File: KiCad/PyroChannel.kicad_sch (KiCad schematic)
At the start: 5 parts, among them Q4 IRLML0030

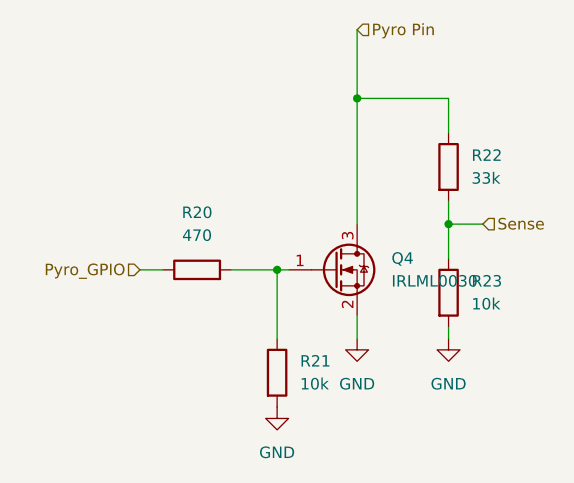
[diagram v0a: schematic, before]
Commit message: Layout started
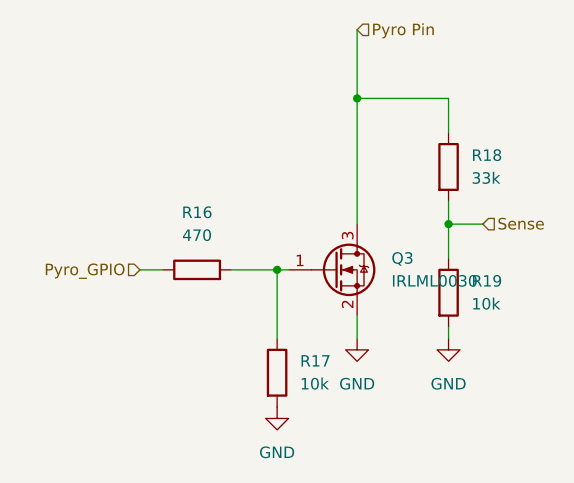
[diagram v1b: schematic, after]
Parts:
- renumbered Q4 to Q3, R20 to R16, R21 to R17, R22 to R18, R23 to R19
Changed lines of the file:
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@@
 		(dnp no)
 		(fields_autoplaced yes)
-		(property "Reference" "#PWR072"
+		(property "Reference" "#PWR069"
 			(at 157.48 107.95 0)
 			(effects
@@
 		(instances
 			(project "Senior Project"
-				(path "/16f8cce7-467e-4342-b55a-00af81cd6f69/4f56c78f-4532-4c9f-be6c-2bbf693c5fca"
+				(path "/16f8cce7-467e-4342-b55a-00af81cd6f69/553e2c15-6dd9-455d-b91b-1c20c70d481b"
+					(reference "#PWR066")
+					(unit 1)
+				)
+				(path "/16f8cce7-467e-4342-b55a-00af81cd6f69/60268ff6-e480-4c50-9139-8340585ef982"
+					(reference "#PWR069")
+					(unit 1)
+				)
+				(path "/16f8cce7-467e-4342-b55a-00af81cd6f69/93da445a-87ee-42db-a7a9-6194d5b9218b"
 					(reference "#PWR072")
-					(unit 1)
-				)
-				(path "/16f8cce7-467e-4342-b55a-00af81cd6f69/528e247e-1625-48b4-9899-73b4b85367ce"
-					(reference "#PWR069")
-					(unit 1)
-				)
-				(path "/16f8cce7-467e-4342-b55a-00af81cd6f69/553e2c15-6dd9-455d-b91b-1c20c70d481b"
-					(reference "#PWR066")
 					(unit 1)
 				)
@@
 		(dnp no)
 		(fields_autoplaced yes)
-		(property "Reference" "#PWR071"
+		(property "Reference" "#PWR068"
 			(at 147.32 107.95 0)
 			(effects
@@
 		(instances
 			(project "Senior Project"
-				(path "/16f8cce7-467e-4342-b55a-00af81cd6f69/4f56c78f-4532-4c9f-be6c-2bbf693c5fca"
+				(path "/16f8cce7-467e-4342-b55a-00af81cd6f69/553e2c15-6dd9-455d-b91b-1c20c70d481b"
+					(reference "#PWR057")
+					(unit 1)
+				)
+				(path "/16f8cce7-467e-4342-b55a-00af81cd6f69/60268ff6-e480-4c50-9139-8340585ef982"
+					(reference "#PWR068")
+					(unit 1)
+				)
+				(path "/16f8cce7-467e-4342-b55a-00af81cd6f69/93da445a-87ee-42db-a7a9-6194d5b9218b"
 					(reference "#PWR071")
-					(unit 1)
-				)
-				(path "/16f8cce7-467e-4342-b55a-00af81cd6f69/528e247e-1625-48b4-9899-73b4b85367ce"
-					(reference "#PWR068")
-					(unit 1)
-				)
-				(path "/16f8cce7-467e-4342-b55a-00af81cd6f69/553e2c15-6dd9-455d-b91b-1c20c70d481b"
-					(reference "#PWR057")
 					(unit 1)
 				)
@@
 		(dnp no)
 		(fields_autoplaced yes)
-		(property "Reference" "R22"
+		(property "Reference" "R18"
 			(at 160.02 81.2799 0)
 			(effects
@@
 		(instances
 			(project "Senior Project"
-				(path "/16f8cce7-467e-4342-b55a-00af81cd6f69/4f56c78f-4532-4c9f-be6c-2bbf693c5fca"
+				(path "/16f8cce7-467e-4342-b55a-00af81cd6f69/553e2c15-6dd9-455d-b91b-1c20c70d481b"
+					(reference "R14")
+					(unit 1)
+				)
+				(path "/16f8cce7-467e-4342-b55a-00af81cd6f69/60268ff6-e480-4c50-9139-8340585ef982"
+					(reference "R18")
+					(unit 1)
+				)
+				(path "/16f8cce7-467e-4342-b55a-00af81cd6f69/93da445a-87ee-42db-a7a9-6194d5b9218b"
 					(reference "R22")
-					(unit 1)
-				)
-				(path "/16f8cce7-467e-4342-b55a-00af81cd6f69/528e247e-1625-48b4-9899-73b4b85367ce"
-					(reference "R18")
-					(unit 1)
-				)
-				(path "/16f8cce7-467e-4342-b55a-00af81cd6f69/553e2c15-6dd9-455d-b91b-1c20c70d481b"
-					(reference "R14")
 					(unit 1)
 				)
@@
 		(dnp no)
 		(fields_autoplaced yes)
-		(property "Reference" "#PWR070"
+		(property "Reference" "#PWR067"
 			(at 138.43 115.57 0)
 			(effects
@@
 		(instances
 			(project "Senior Project"
-				(path "/16f8cce7-467e-4342-b55a-00af81cd6f69/4f56c78f-4532-4c9f-be6c-2bbf693c5fca"
+				(path "/16f8cce7-467e-4342-b55a-00af81cd6f69/553e2c15-6dd9-455d-b91b-1c20c70d481b"
+					(reference "#PWR056")
+					(unit 1)
+				)
+				(path "/16f8cce7-467e-4342-b55a-00af81cd6f69/60268ff6-e480-4c50-9139-8340585ef982"
+					(reference "#PWR067")
+					(unit 1)
+				)
+				(path "/16f8cce7-467e-4342-b55a-00af81cd6f69/93da445a-87ee-42db-a7a9-6194d5b9218b"
 					(reference "#PWR070")
-					(unit 1)
-				)
-				(path "/16f8cce7-467e-4342-b55a-00af81cd6f69/528e247e-1625-48b4-9899-73b4b85367ce"
-					(reference "#PWR067")
-					(unit 1)
-				)
-				(path "/16f8cce7-467e-4342-b55a-00af81cd6f69/553e2c15-6dd9-455d-b91b-1c20c70d481b"
-					(reference "#PWR056")
 					(unit 1)
 				)
@@
 		(dnp no)
 		(fields_autoplaced yes)
-		(property "Reference" "R20"
+		(property "Reference" "R16"
 			(at 129.54 87.63 90)
 			(effects
@@
 		(instances
 			(project "Senior Project"
-				(path "/16f8cce7-467e-4342-b55a-00af81cd6f69/4f56c78f-4532-4c9f-be6c-2bbf693c5fca"
+				(path "/16f8cce7-467e-4342-b55a-00af81cd6f69/553e2c15-6dd9-455d-b91b-1c20c70d481b"
+					(reference "R12")
+					(unit 1)
+				)
+				(path "/16f8cce7-467e-4342-b55a-00af81cd6f69/60268ff6-e480-4c50-9139-8340585ef982"
+					(reference "R16")
+					(unit 1)
+				)
+				(path "/16f8cce7-467e-4342-b55a-00af81cd6f69/93da445a-87ee-42db-a7a9-6194d5b9218b"
 					(reference "R20")
-					(unit 1)
-				)
-				(path "/16f8cce7-467e-4342-b55a-00af81cd6f69/528e247e-1625-48b4-9899-73b4b85367ce"
-					(reference "R16")
-					(unit 1)
-				)
-				(path "/16f8cce7-467e-4342-b55a-00af81cd6f69/553e2c15-6dd9-455d-b91b-1c20c70d481b"
-					(reference "R12")
 					(unit 1)
 				)
@@
 		(dnp no)
 		(fields_autoplaced yes)
-		(property "Reference" "Q4"
+		(property "Reference" "Q3"
 			(at 151.13 92.7099 0)
 			(effects
@@
 		(instances
 			(project "Senior Project"
-				(path "/16f8cce7-467e-4342-b55a-00af81cd6f69/4f56c78f-4532-4c9f-be6c-2bbf693c5fca"
+				(path "/16f8cce7-467e-4342-b55a-00af81cd6f69/553e2c15-6dd9-455d-b91b-1c20c70d481b"
+					(reference "Q2")
+					(unit 1)
+				)
+				(path "/16f8cce7-467e-4342-b55a-00af81cd6f69/60268ff6-e480-4c50-9139-8340585ef982"
+					(reference "Q3")
+					(unit 1)
+				)
+				(path "/16f8cce7-467e-4342-b55a-00af81cd6f69/93da445a-87ee-42db-a7a9-6194d5b9218b"
 					(reference "Q4")
-					(unit 1)
-				)
-				(path "/16f8cce7-467e-4342-b55a-00af81cd6f69/528e247e-1625-48b4-9899-73b4b85367ce"
-					(reference "Q3")
-					(unit 1)
-				)
-				(path "/16f8cce7-467e-4342-b55a-00af81cd6f69/553e2c15-6dd9-455d-b91b-1c20c70d481b"
-					(reference "Q2")
 					(unit 1)
 				)
@@
 		(dnp no)
 		(fields_autoplaced yes)
-		(property "Reference" "R21"
+		(property "Reference" "R17"
 			(at 140.97 104.1399 0)
 			(effects
@@
 		(instances
 			(project "Senior Project"
-				(path "/16f8cce7-467e-4342-b55a-00af81cd6f69/4f56c78f-4532-4c9f-be6c-2bbf693c5fca"
+				(path "/16f8cce7-467e-4342-b55a-00af81cd6f69/553e2c15-6dd9-455d-b91b-1c20c70d481b"
+					(reference "R13")
+					(unit 1)
+				)
+				(path "/16f8cce7-467e-4342-b55a-00af81cd6f69/60268ff6-e480-4c50-9139-8340585ef982"
+					(reference "R17")
+					(unit 1)
+				)
+				(path "/16f8cce7-467e-4342-b55a-00af81cd6f69/93da445a-87ee-42db-a7a9-6194d5b9218b"
 					(reference "R21")
-					(unit 1)
-				)
-				(path "/16f8cce7-467e-4342-b55a-00af81cd6f69/528e247e-1625-48b4-9899-73b4b85367ce"
-					(reference "R17")
-					(unit 1)
-				)
-				(path "/16f8cce7-467e-4342-b55a-00af81cd6f69/553e2c15-6dd9-455d-b91b-1c20c70d481b"
-					(reference "R13")
 					(unit 1)
 				)
@@
 		(dnp no)
 		(fields_autoplaced yes)
-		(property "Reference" "R23"
+		(property "Reference" "R19"
 			(at 160.02 95.2499 0)
 			(effects
@@
 		(instances
 			(project "Senior Project"
-				(path "/16f8cce7-467e-4342-b55a-00af81cd6f69/4f56c78f-4532-4c9f-be6c-2bbf693c5fca"
+				(path "/16f8cce7-467e-4342-b55a-00af81cd6f69/553e2c15-6dd9-455d-b91b-1c20c70d481b"
+					(reference "R15")
+					(unit 1)
+				)
+				(path "/16f8cce7-467e-4342-b55a-00af81cd6f69/60268ff6-e480-4c50-9139-8340585ef982"
+					(reference "R19")
+					(unit 1)
+				)
+				(path "/16f8cce7-467e-4342-b55a-00af81cd6f69/93da445a-87ee-42db-a7a9-6194d5b9218b"
 					(reference "R23")
 					(unit 1)
 				)
-				(path "/16f8cce7-467e-4342-b55a-00af81cd6f69/528e247e-1625-48b4-9899-73b4b85367ce"
-					(reference "R19")
-					(unit 1)
-				)
-				(path "/16f8cce7-467e-4342-b55a-00af81cd6f69/553e2c15-6dd9-455d-b91b-1c20c70d481b"
-					(reference "R15")
-					(unit 1)
-				)
